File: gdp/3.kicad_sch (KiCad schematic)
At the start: 9 parts, among them IC22 PAL16L8, IC23 EF9367, IC24 PAL10L8, IC49 PAL16R4

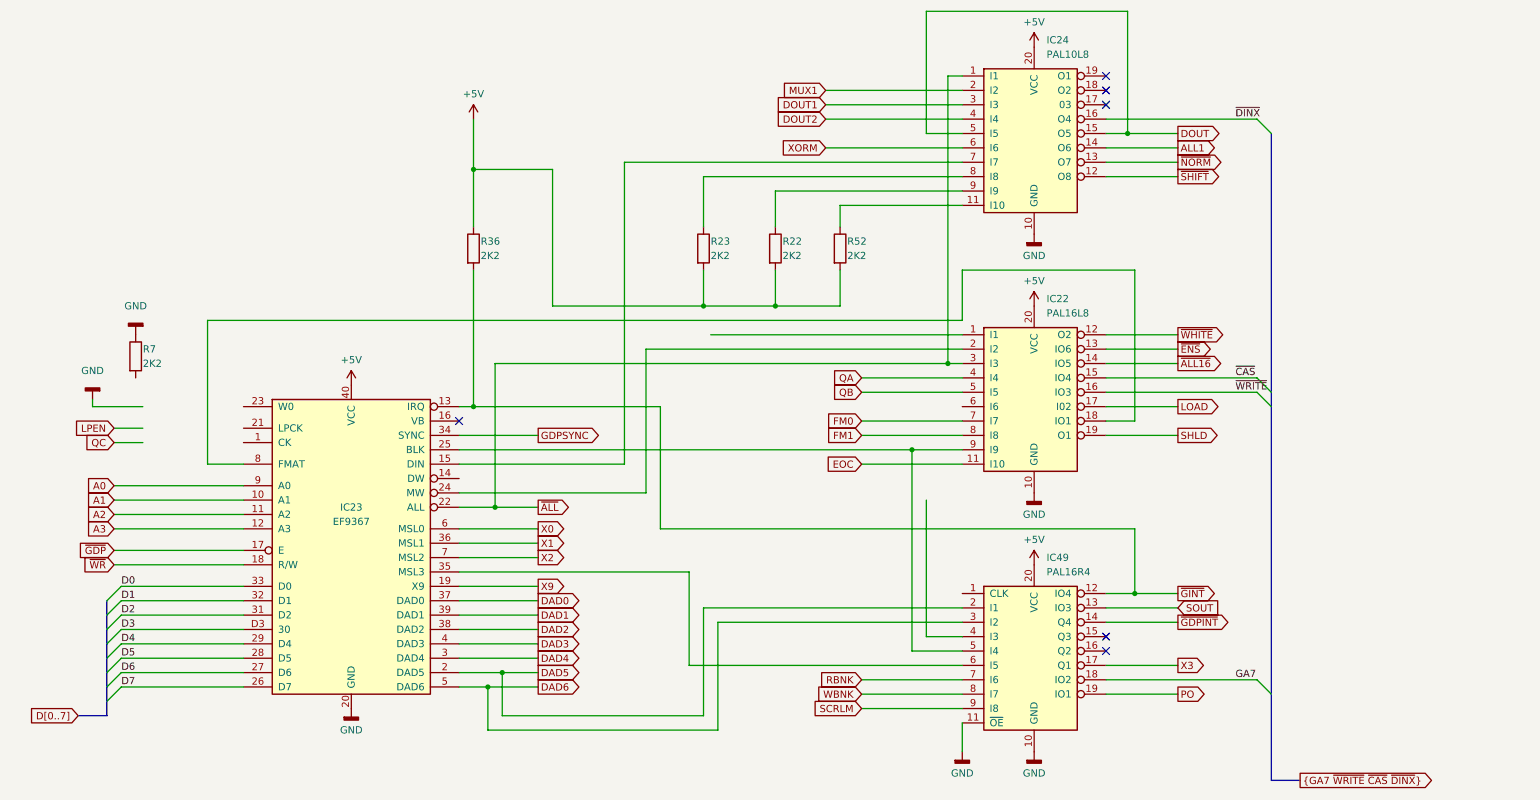
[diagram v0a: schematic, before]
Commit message: Small fixes
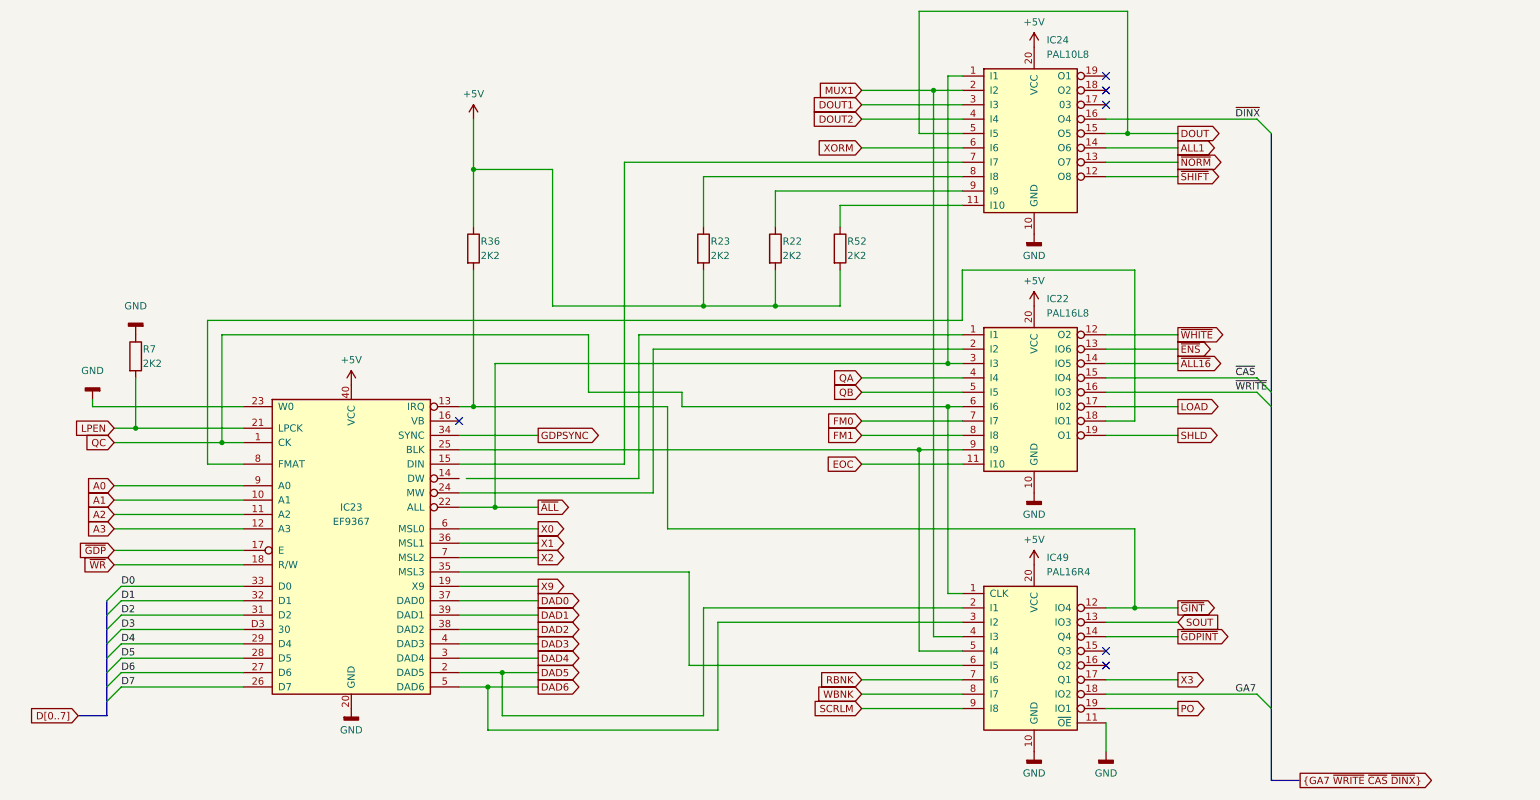
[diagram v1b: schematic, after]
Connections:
- net GND: now also IC23.23 (W0)
- net LPEN: now also IC23.21 (LPCK), R7.2
- net MUX1: now also IC49.4 (I3)
- net QC: now also IC22.6 (I6), IC23.1 (CK), IC49.1 (CLK)
